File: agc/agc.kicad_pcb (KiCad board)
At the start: 2 copper layers, 72.4 x 59.1 mm, 63 parts, among them J5 SIL10, K1 TR, K10 HVMON, K11 HVMON, K2 TR, K3 VIN, K4 VOUT_TR, K5 TR, K6 TR, K7 HVMON, K8 TR, K9 TR, P4 CONN_8X2, P9 COUPLED_TEST, U10 74AHC1G04, U11 74AHC1G04, U12 78SRH-5/2-C, U6 74AHC1G04, U7 ISL3281E, U9 LTC2914-2

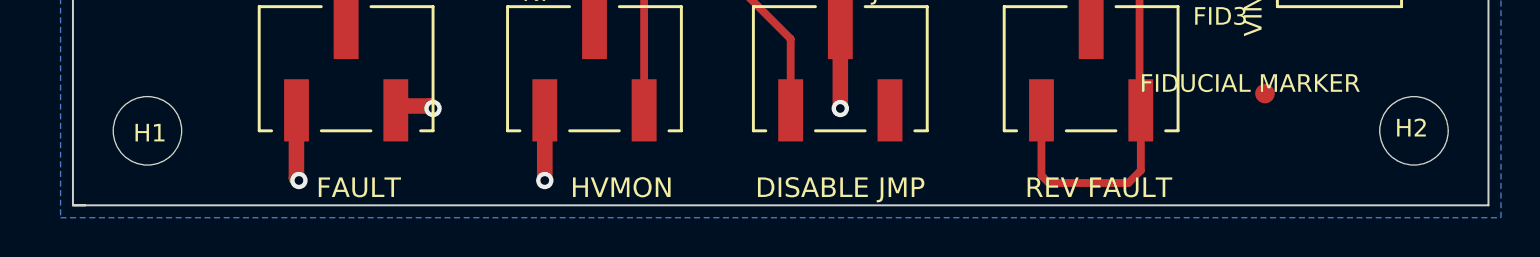
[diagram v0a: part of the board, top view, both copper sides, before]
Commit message: DFM changes..
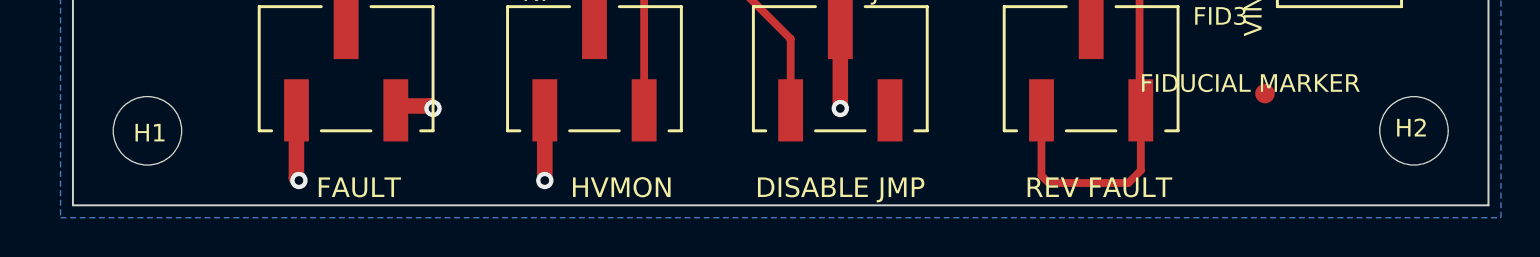
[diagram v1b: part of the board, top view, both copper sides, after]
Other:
- outline, holes or cut-outs redrawn
